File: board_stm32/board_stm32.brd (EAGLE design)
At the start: 160 x 100 mm, 8 parts, among them IC2 NE555, T1 BC547

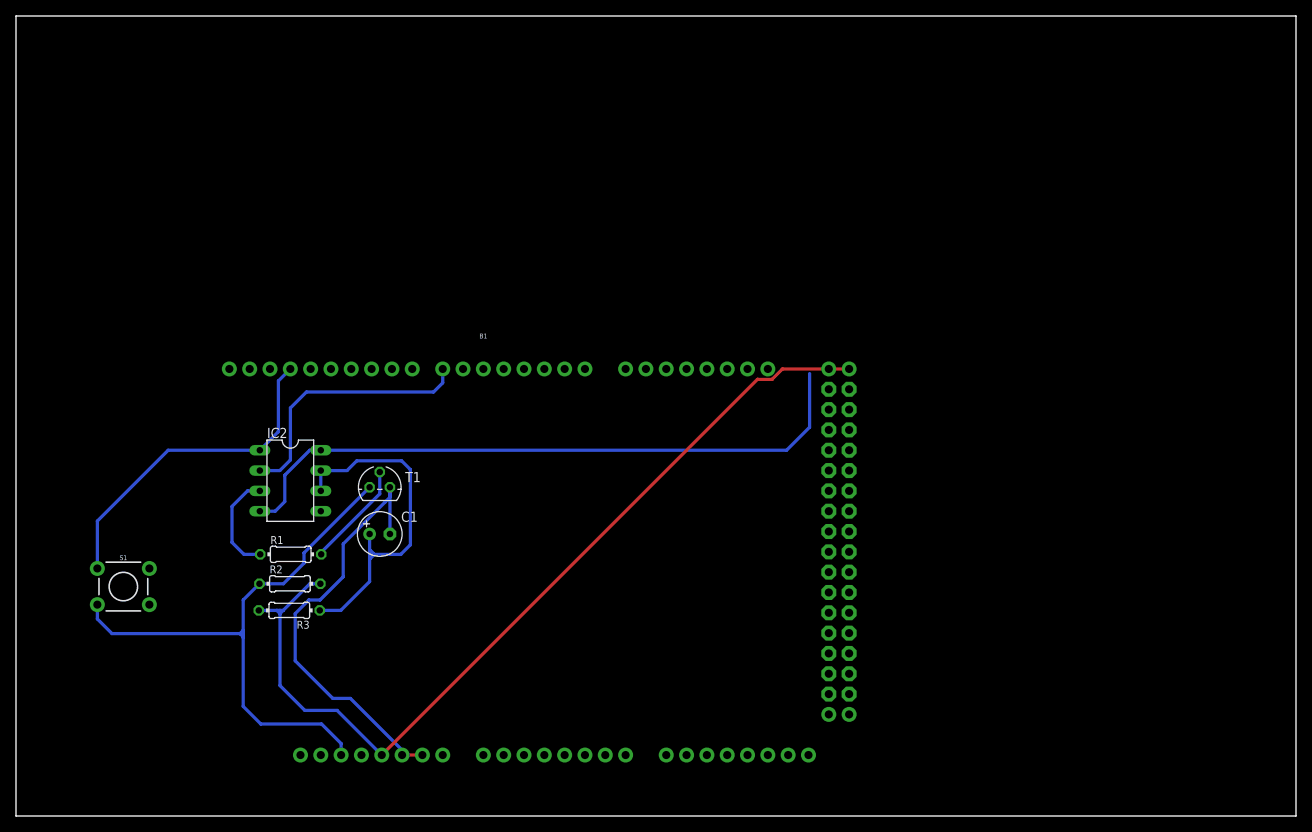
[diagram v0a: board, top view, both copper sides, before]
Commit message: update schematic and board, add .gitignore
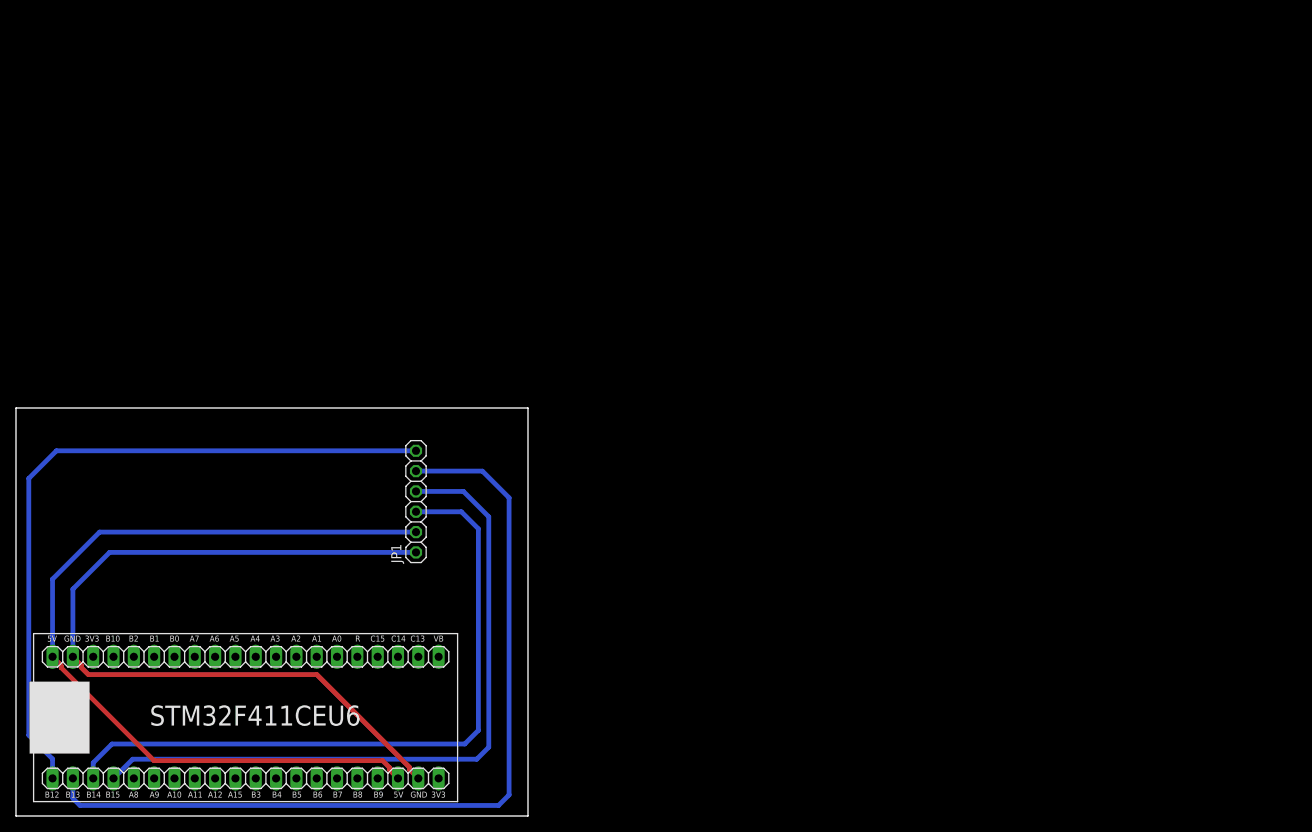
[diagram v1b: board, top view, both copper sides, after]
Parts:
- removed B1: ARDUINO_MEGA_R3FULL, SparkFun-Boards:ARDUINO_MEGA_NO_SILK
- removed C1: (no value), rcl:E2,5-6
- removed IC2: NE555, st-microelectronics:DIL-08
- removed R1, R2, R3: (no value), rcl:0204/7
- removed S1: MOMENTARY-SWITCH-SPST-PTH-6.0MM, SparkFun-Switches:TACTILE_SWITCH_PTH_6.0MM
- removed T1: BC547, transistor:TO92
- added JP1: (no value), adafruit:1X06
- added U$1: STM32F411CEU6, STM32F411CEU6:STM32F411CEU6
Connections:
- removed net 5V: B1.5V, B1.5V@1, B1.5V@2, IC2.4, IC2.8, R2.2, R3.2
- removed net N$1: C1.+, IC2.6, IC2.7, R3.1
- removed net N$2: IC2.3, R1.1
- removed net N$3: R1.2, T1.2
- removed net RST: B1.RESET, R2.1, S1.3, T1.3
- removed net RST_GPIO: B1.7, IC2.2
- new net CS: JP1.6, U$1.B12
- new net MISO: JP1.3, U$1.B14
- new net MOSI: JP1.4, U$1.B15
- new net SCK: JP1.5, U$1.B13
- new net VCC: JP1.2, U$1.5V, U$1.5V_2
- net GND: now also JP1.1, U$1.GND, U$1.GND2; no longer B1.GND, B1.GND@1, B1.GND@3, B1.GND@4, C1.-, IC2.1, S1.1, T1.1
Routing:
- net 5V: track 196.0 -> 0.00 mm
- net SCK: track 0.00 -> 108.1 mm
- net VCC: track 0.00 -> 107.4 mm
- net CS: track 0.00 -> 88.6 mm
- net MOSI: track 0.00 -> 87.7 mm
- net MISO: track 0.00 -> 85.7 mm
- net RST: track 73.2 -> 0.00 mm
- net N$1: track 45.0 -> 0.00 mm
- net RST_GPIO: track 32.9 -> 0.00 mm
- net N$3: track 13.3 -> 0.00 mm
- net N$2: track 12.9 -> 0.00 mm
- net GND: track 96.0 -> 103.1 mm
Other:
- board size 160 x 100 mm -> 64 x 51 mm

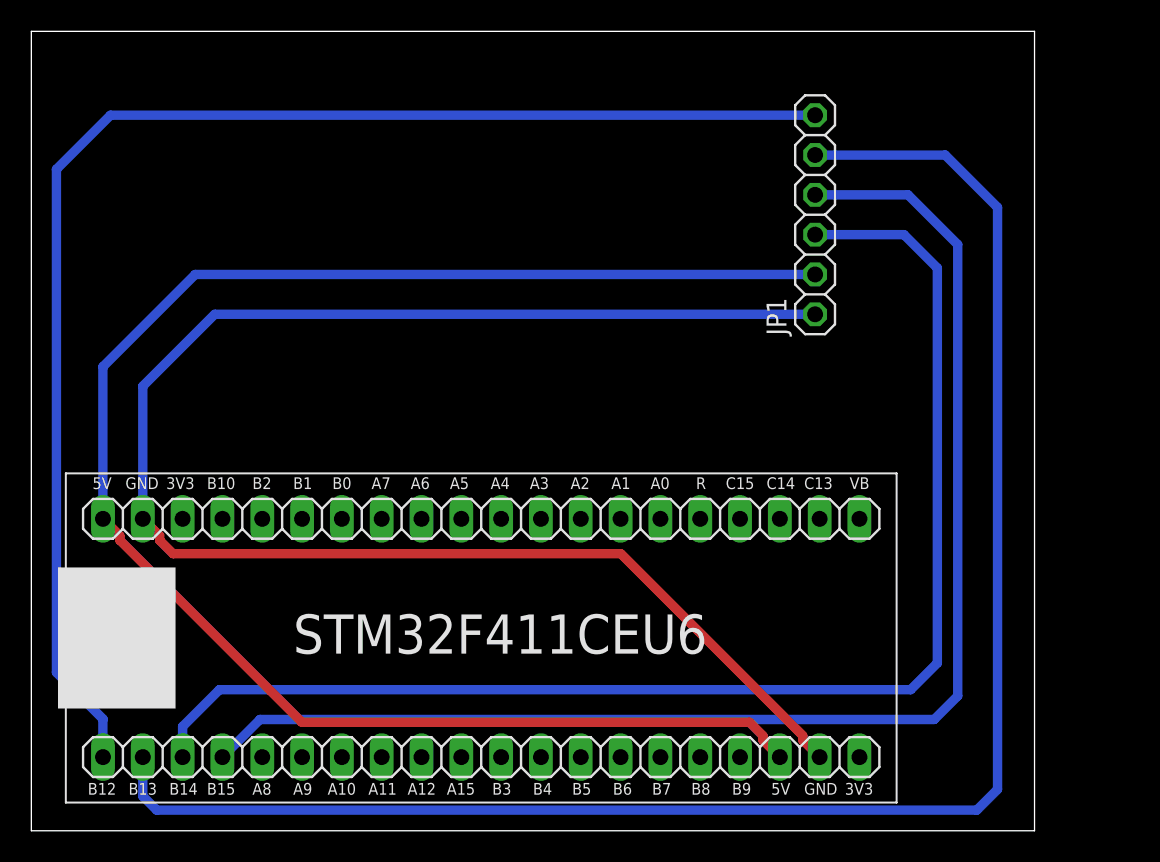
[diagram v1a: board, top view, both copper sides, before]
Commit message: redesign PCB
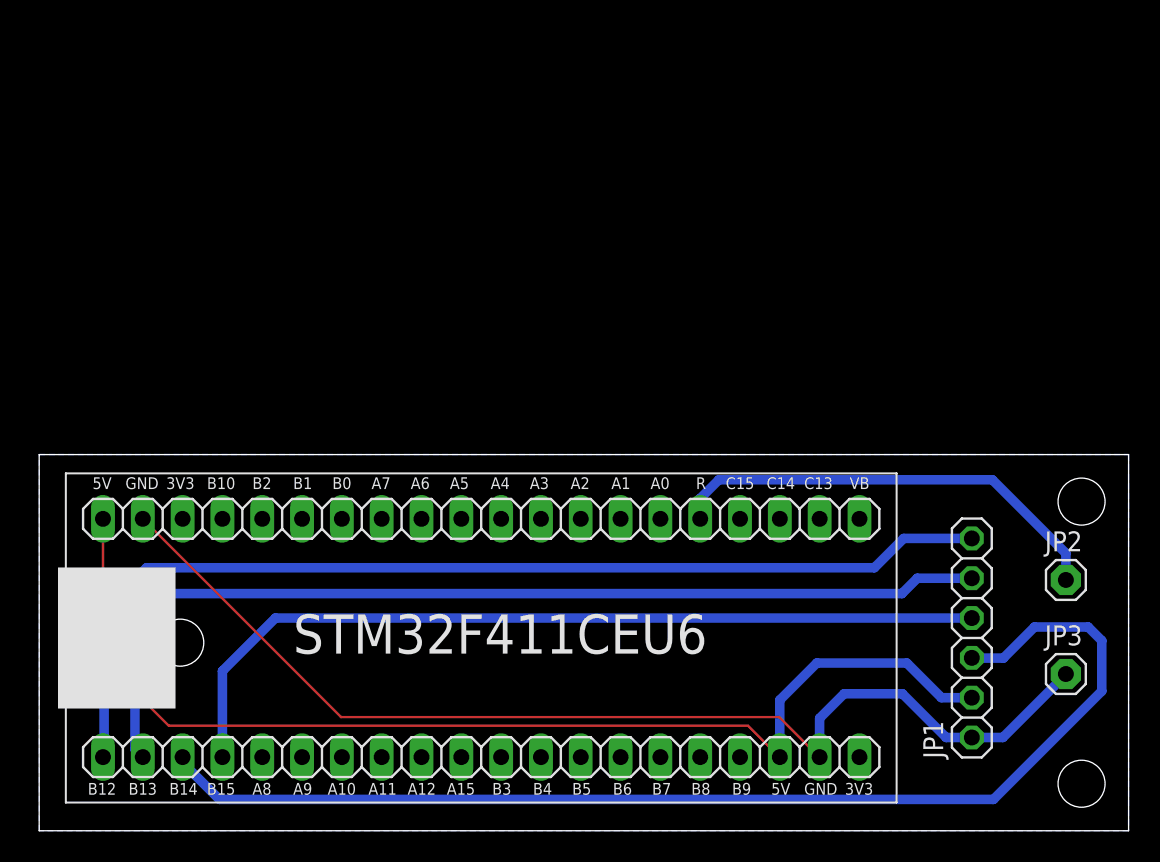
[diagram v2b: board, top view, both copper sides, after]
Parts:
- added JP2, JP3: (no value), adafruit:1X01
- moved JP1 28.8 mm to (60.0, 12.3)
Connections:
- new net N$1: JP2.1, U$1.R
- net GND: now also JP3.1
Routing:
- net SCK: track 108.1 -> 63.5 mm
- net VCC: track 107.4 -> 72.5 mm
- net MOSI: track 87.7 -> 54.7 mm
- net GND: track 103.1 -> 71.2 mm
- net N$1: track 0.00 -> 28.8 mm
- net CS: track 88.6 -> 66.7 mm
- net MISO: track 85.7 -> 75.5 mm
- added copper zone on layer 16, net GND
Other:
- board size 64 x 51 mm -> 69.5 x 24 mm
